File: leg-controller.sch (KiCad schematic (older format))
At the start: 15 parts, among them J1 Conn_01x02, J2 Conn_01x03, U1 LD1117S33TR_SOT223, U2 ATmega644P-20AU, Y1 12MHz

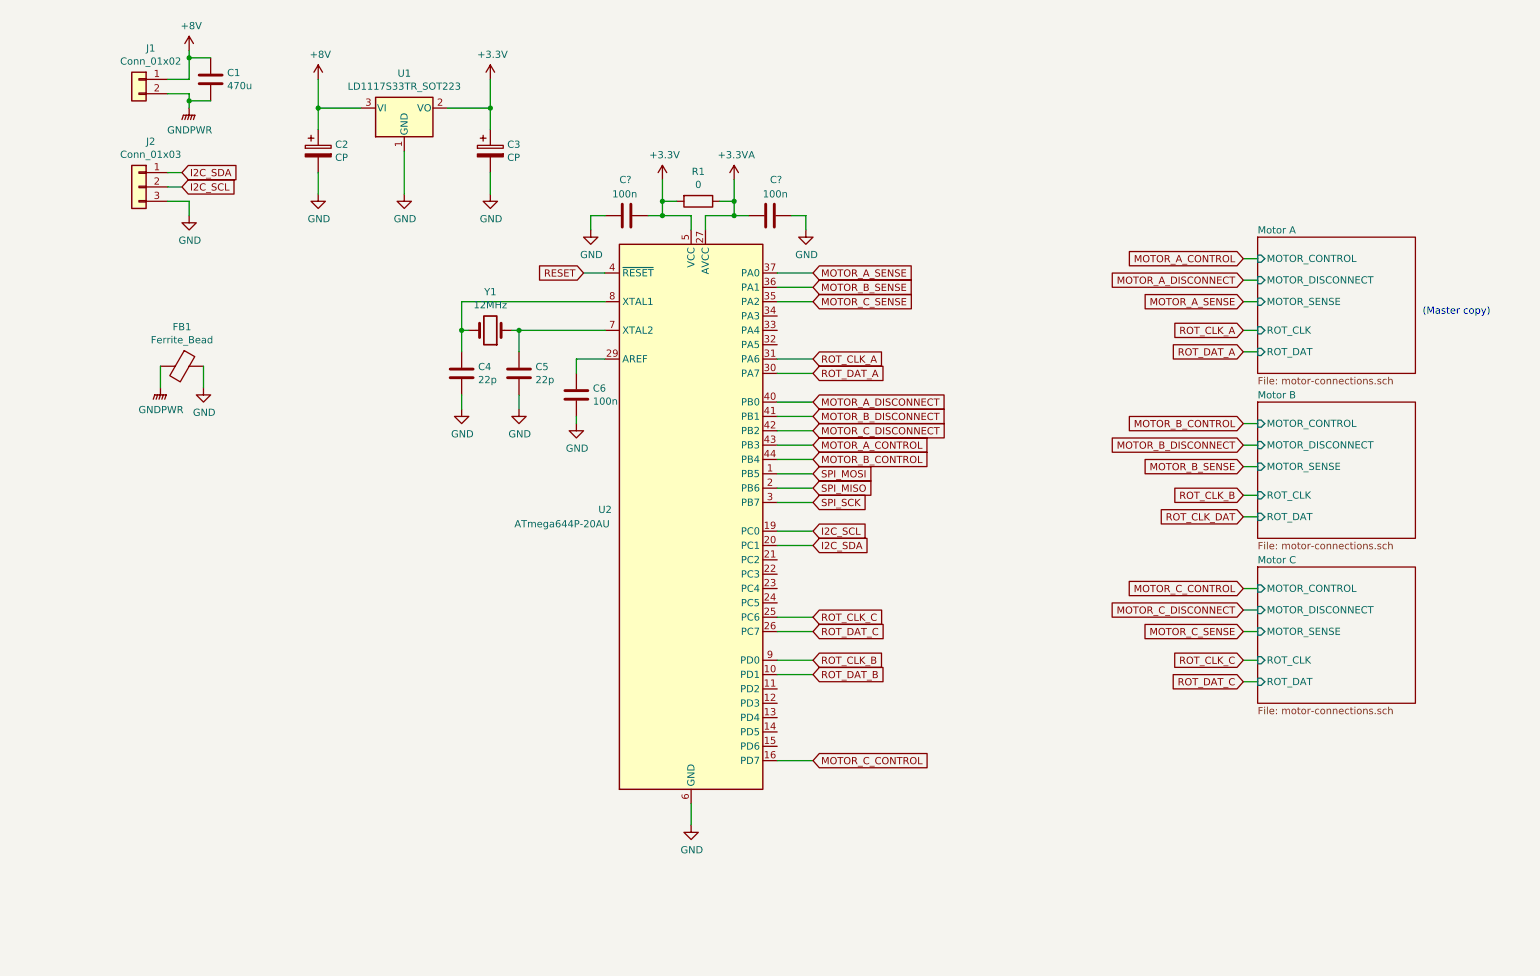
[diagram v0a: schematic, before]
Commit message: Various changes
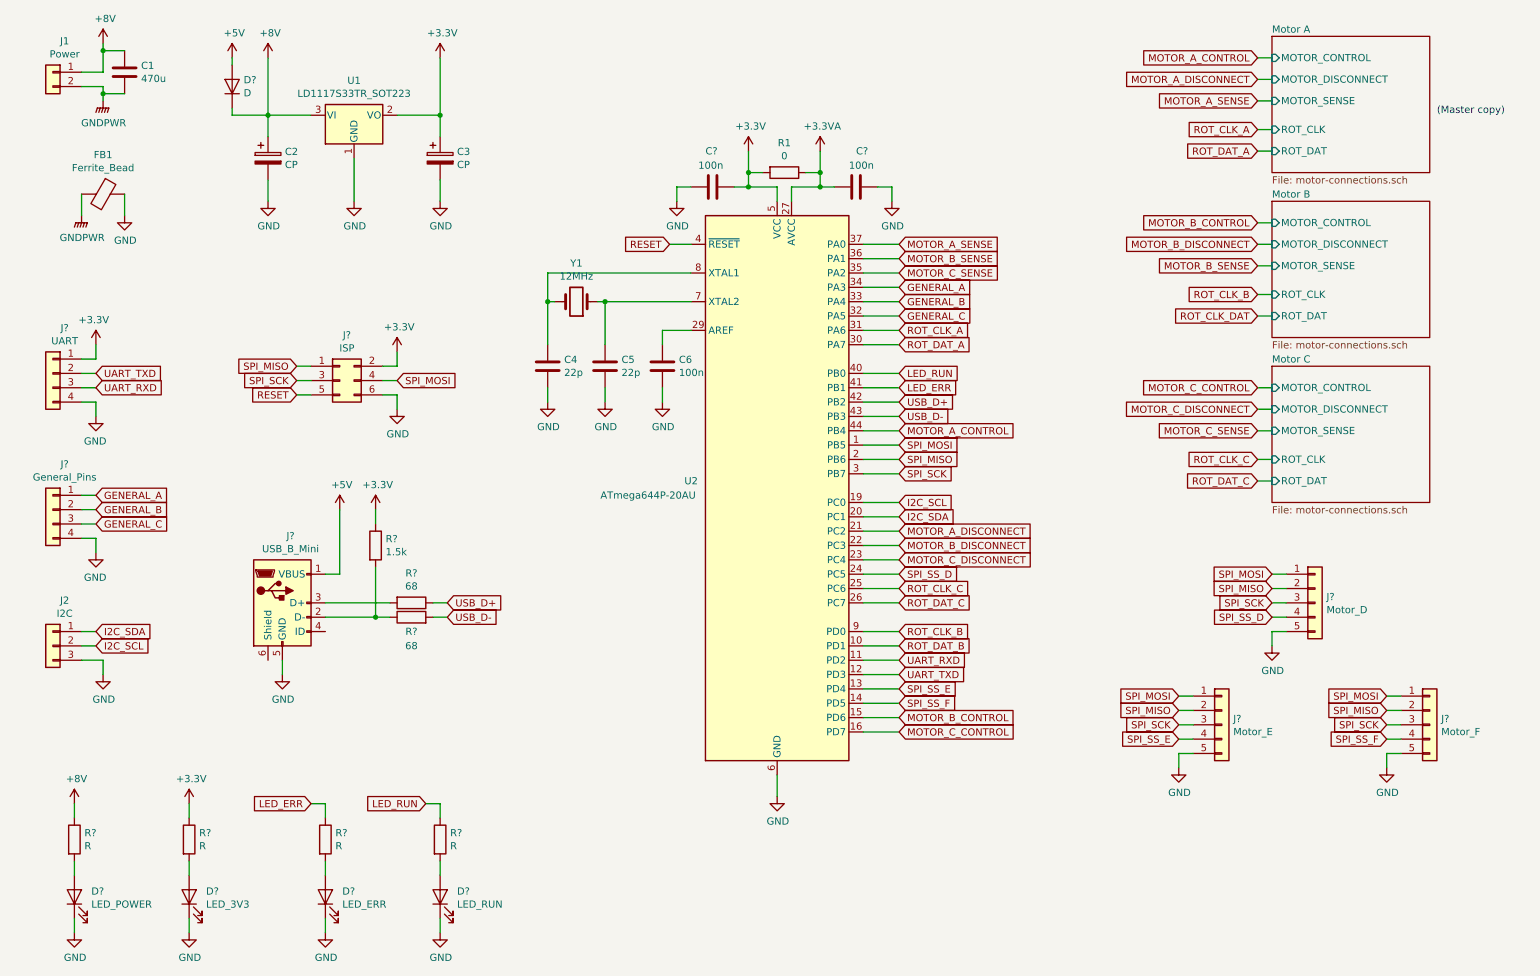
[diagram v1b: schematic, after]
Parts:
- added D?: LED_RUN, symbol Device:LED
- added D?: LED_POWER, symbol Device:LED
- added D?: LED_3V3, symbol Device:LED
- added D?: LED_ERR, symbol Device:LED
- added D?: D, symbol Device:D
- added J?: Motor_D, symbol Connector_Generic:Conn_01x05
- added J?: Motor_F, symbol Connector_Generic:Conn_01x05
- added J?: Motor_E, symbol Connector_Generic:Conn_01x05
- added J?: ISP, symbol Connector_Generic:Conn_02x03_Odd_Even
- added J?: UART, symbol Connector_Generic:Conn_01x04
- added J?: General_Pins, symbol Connector_Generic:Conn_01x04
- added J?: USB_B_Mini, symbol Connector:USB_B_Mini
- added R? (x4): R, symbol Device:R
- added R? (x2): 68, symbol Device:R
- added R?: 1.5k, symbol Device:R
- J1: value Conn_01x02 -> Power
- J2: value Conn_01x03 -> I2C
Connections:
- net +3V3: now also J?.1 (Pin_1), J?.2 (Pin_2), R?.1, R?.1
- net +8V: now also D?.1 (K), R?.1
- net GND: now also D?.1 (K), D?.1 (K), D?.1 (K), D?.1 (K), J?.4 (Pin_4), J?.4 (Pin_4), J?.5 (GND), J?.5 (Pin_5), J?.5 (Pin_5), J?.5 (Pin_5), J?.6 (Pin_6)
- net MOTOR_A_CONTROL: now also U2.44 (PB4); no longer U2.43 (PB3)
- net MOTOR_A_DISCONNECT: now also U2.21 (PC2); no longer U2.40 (PB0)
- net MOTOR_B_CONTROL: now also U2.15 (PD6); no longer U2.44 (PB4)
- net MOTOR_B_DISCONNECT: now also U2.22 (PC3); no longer U2.41 (PB1)
- net MOTOR_C_DISCONNECT: now also U2.23 (PC4); no longer U2.42 (PB2)
- net RESET: now also J?.5 (Pin_5)
- net SPI_MISO: now also J?.1 (Pin_1), J?.2 (Pin_2), J?.2 (Pin_2), J?.2 (Pin_2)
- net SPI_MOSI: now also J?.1 (Pin_1), J?.1 (Pin_1), J?.1 (Pin_1), J?.4 (Pin_4)
- net SPI_SCK: now also J?.3 (Pin_3), J?.3 (Pin_3), J?.3 (Pin_3), J?.3 (Pin_3)
- net UART_RXD: now reaches U2.11 (PD2)
- net UART_RXD: now also J?.3 (Pin_3)
- net UART_TXD: now reaches U2.12 (PD3)
- net UART_TXD: now also J?.2 (Pin_2)
- net SPI_SS_E: now reaches U2.13 (PD4)
- net SPI_SS_E: now also J?.4 (Pin_4)
- net SPI_SS_F: now reaches U2.14 (PD5)
- net SPI_SS_F: now also J?.4 (Pin_4)
- net SPI_SS_D: now reaches U2.24 (PC5)
- net SPI_SS_D: now also J?.4 (Pin_4)
- net GENERAL_C: now reaches U2.32 (PA5)
- net GENERAL_C: now also J?.3 (Pin_3)
- net GENERAL_B: now reaches U2.33 (PA4)
- net GENERAL_B: now also J?.2 (Pin_2)
- net GENERAL_A: now reaches U2.34 (PA3)
- net GENERAL_A: now also J?.1 (Pin_1)
- new net: D?.2 (A), R?.2 (x4)
- new net: J?.2 (D-), R?.1, R?.2
- new net: J?.3 (D+), R?.2
- new net +5V: D?.2 (A), J?.1 (VBUS)
- new net LED_ERR: R?.1, U2.41 (PB1)
- new net LED_RUN: R?.1, U2.40 (PB0)
- new net USB_D+: R?.1, U2.42 (PB2)
- new net USB_D-: R?.2, U2.43 (PB3)
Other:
- moved on the sheet: C1, C2, C3, C4, C5, C6, C?, FB1, J1, J2, R1, U1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

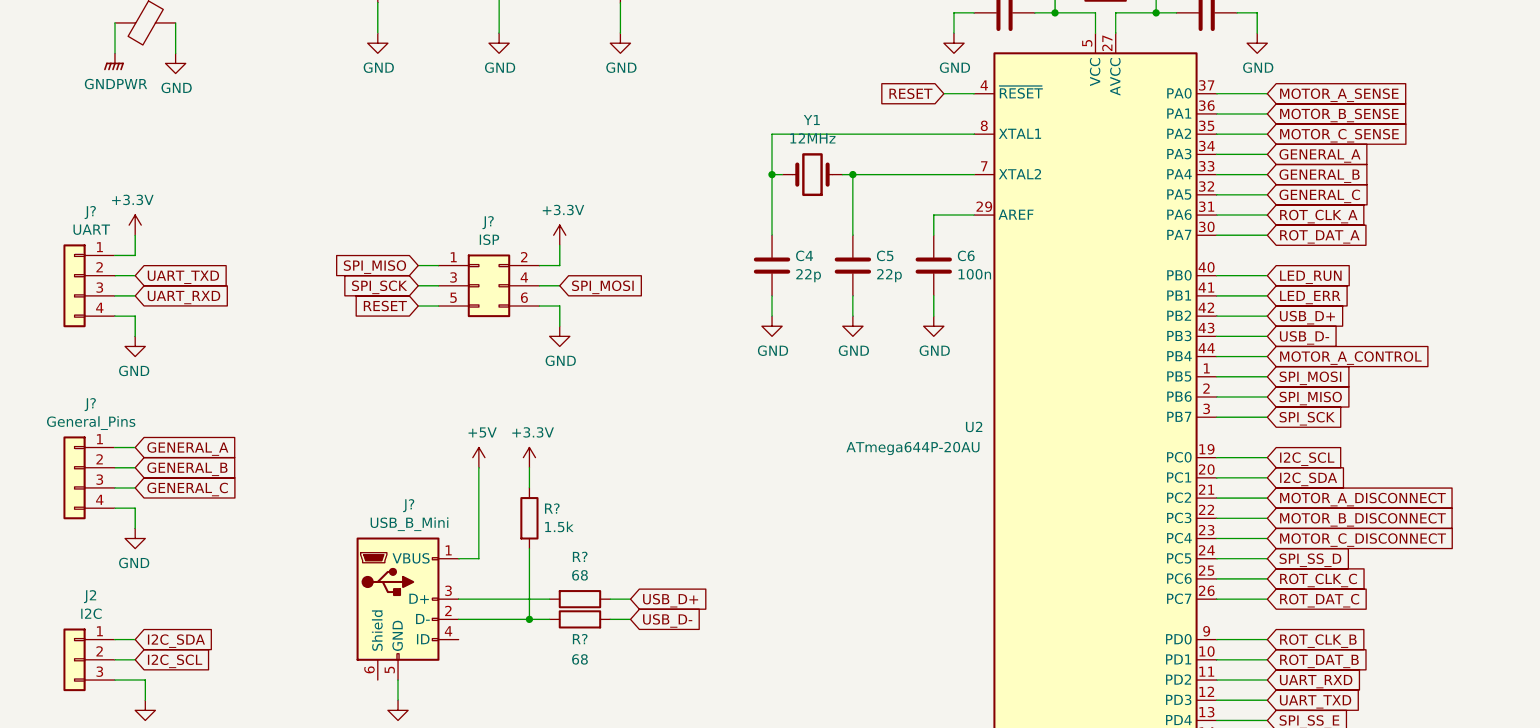
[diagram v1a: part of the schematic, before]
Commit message: Various changes.
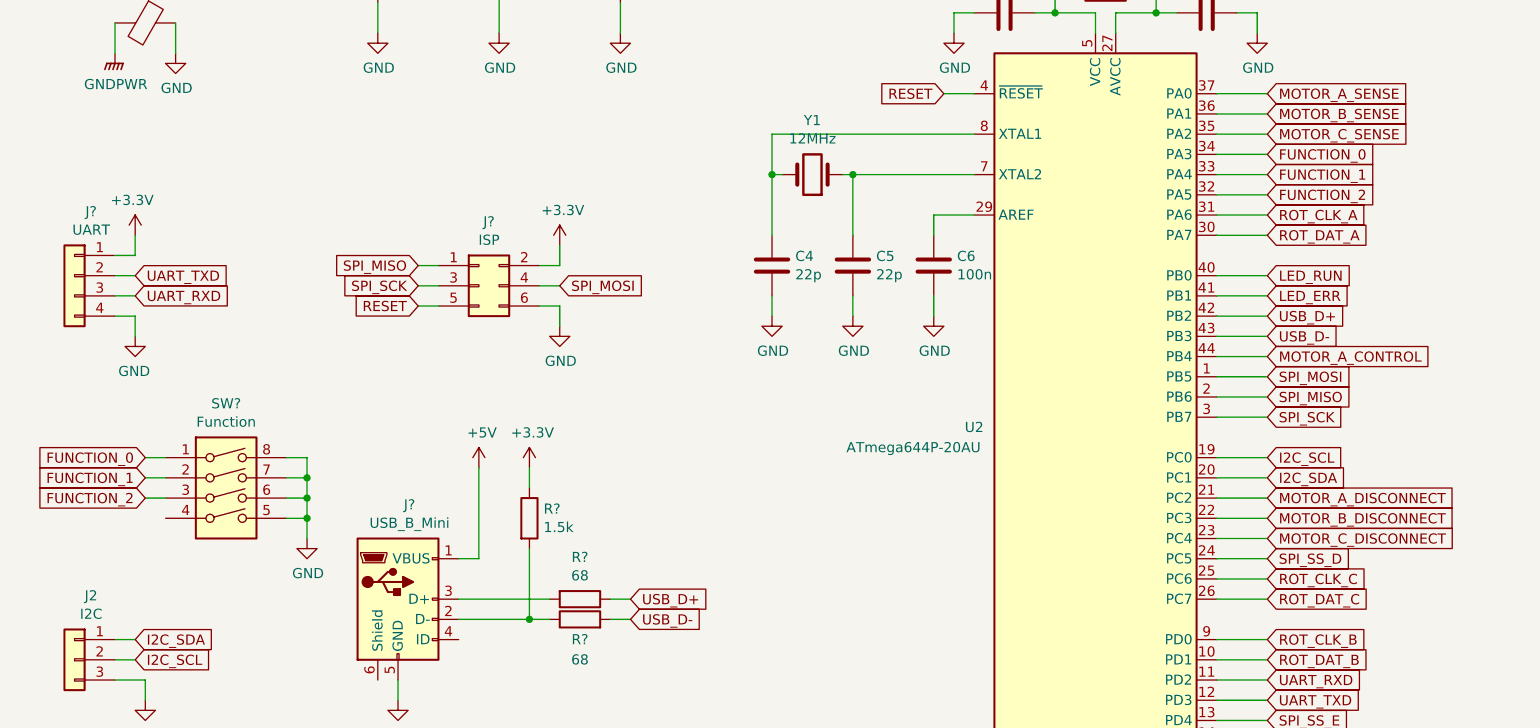
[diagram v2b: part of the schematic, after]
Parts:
- removed J?: General_Pins, symbol Connector_Generic:Conn_01x04
- added SW?: Function, symbol Switch:SW_DIP_x04
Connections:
- net GND: now also SW?.5, SW?.6, SW?.7, SW?.8
- net GENERAL_A renamed FUNCTION_0
- net FUNCTION_0: now also SW?.1
- net GENERAL_B renamed FUNCTION_1
- net FUNCTION_1: now also SW?.2
- net GENERAL_C renamed FUNCTION_2
- net FUNCTION_2: now also SW?.3
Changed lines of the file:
@@
 Wire Wire Line
 	3150 3250 3250 3250
-Text GLabel 1150 4050 2    50   Input ~ 0
-GENERAL_A
-Text GLabel 1150 4150 2    50   Input ~ 0
-GENERAL_B
-Text GLabel 1150 4250 2    50   Input ~ 0
-GENERAL_C
-Wire Wire Line
-	1150 4050 1050 4050
-Wire Wire Line
-	1050 4150 1150 4150
-Wire Wire Line
-	1150 4250 1050 4250
-$Comp
-L power:GND #PWR?
-U 1 1 61C68C47
-P 1150 4450
-F 0 "#PWR?" H 1150 4200 50  0001 C CNN
-F 1 "GND" H 1155 4277 50  0000 C CNN
-F 2 "" H 1150 4450 50  0001 C CNN
-F 3 "" H 1150 4450 50  0001 C CNN
-	1    1150 4450
-	-1   0    0    -1
-$EndComp
-Wire Wire Line
-	1150 4450 1150 4350
-Wire Wire Line
-	1150 4350 1050 4350
 $Comp
 L power:+5V #PWR?
@@
 $Comp
 L Connector_Generic:Conn_01x04 J?
-U 1 1 61C5169E
-P 850 4150
-F 0 "J?" H 768 4467 50  0000 C CNN
-F 1 "General_Pins" H 768 4376 50  0000 C CNN
-F 2 "" H 850 4150 50  0001 C CNN
-F 3 "~" H 850 4150 50  0001 C CNN
-	1    850  4150
-	-1   0    0    -1
-$EndComp
-$Comp
-L power:GND #PWR04
-U 1 1 6179673C
-P 1200 5300
-F 0 "#PWR04" H 1200 5050 50  0001 C CNN
-F 1 "GND" H 1205 5127 50  0000 C CNN
-F 2 "" H 1200 5300 50  0001 C CNN
-F 3 "" H 1200 5300 50  0001 C CNN
-	1    1200 5300
-	1    0    0    -1
-$EndComp
-Wire Wire Line
-	1200 5200 1200 5300
-Wire Wire Line
-	1050 5200 1200 5200
-Wire Wire Line
-	1050 5000 1150 5000
-Wire Wire Line
-	1050 5100 1150 5100
-Text GLabel 1150 5000 2    50   Input ~ 0
-I2C_SDA
-Text GLabel 1150 5100 2    50   Input ~ 0
-I2C_SCL
-$Comp
-L Connector_Generic:Conn_01x03 J2
-U 1 1 61793AA3
-P 850 5100
-F 0 "J2" H 768 5417 50  0000 C CNN
-F 1 "I2C" H 768 5326 50  0000 C CNN
-F 2 "" H 850 5100 50  0001 C CNN
-F 3 "~" H 850 5100 50  0001 C CNN
-	1    850  5100
-	-1   0    0    -1
-$EndComp
-$Comp
-L Connector_Generic:Conn_01x04 J?
 U 1 1 61B3D105
 P 850 3200
@@
 Wire Wire Line
 	1050 3200 1150 3200
-$Comp
-L Connector:USB_B_Mini J?
-U 1 1 61C85C74
-P 2450 4800
-F 0 "J?" H 2507 5267 50  0000 C CNN
-F 1 "USB_B_Mini" H 2507 5176 50  0000 C CNN
-F 2 "" H 2600 4750 50  0001 C CNN
-F 3 "~" H 2600 4750 50  0001 C CNN
-	1    2450 4800
-	1    0    0    -1
-$EndComp
-$Comp
-L Device:R R?
-U 1 1 61C9C39E
-P 3350 4800
-F 0 "R?" V 3143 4800 50  0000 C CNN
-F 1 "68" V 3234 4800 50  0000 C CNN
-F 2 "" V 3280 4800 50  0001 C CNN
-F 3 "~" H 3350 4800 50  0001 C CNN
-	1    3350 4800
-	0    1    1    0
-$EndComp
-$Comp
-L Device:R R?
-U 1 1 61C9D08A
-P 3350 4900
-F 0 "R?" V 3250 4900 50  0000 C CNN
-F 1 "68" V 3150 4900 50  0000 C CNN
-F 2 "" V 3280 4900 50  0001 C CNN
-F 3 "~" H 3350 4900 50  0001 C CNN
-	1    3350 4900
-	0    -1   -1   0
-$EndComp
-$Comp
-L Device:R R?
-U 1 1 61CB53AC
-P 3100 4400
-F 0 "R?" H 3170 4446 50  0000 L CNN
-F 1 "1.5k" H 3170 4355 50  0000 L CNN
-F 2 "" V 3030 4400 50  0001 C CNN
-F 3 "~" H 3100 4400 50  0001 C CNN
-	1    3100 4400
-	1    0    0    -1
-$EndComp
-Wire Wire Line
-	3100 4550 3100 4900
-Connection ~ 3100 4900
-Wire Wire Line
-	3100 4900 3200 4900
-$Comp
-L power:+3.3V #PWR?
-U 1 1 61CBCED0
-P 3100 4150
-F 0 "#PWR?" H 3100 4000 50  0001 C CNN
-F 1 "+3.3V" H 3115 4323 50  0000 C CNN
-F 2 "" H 3100 4150 50  0001 C CNN
-F 3 "" H 3100 4150 50  0001 C CNN
-	1    3100 4150
-	1    0    0    -1
-$EndComp
-Wire Wire Line
-	3100 4150 3100 4250
-$Comp
-L power:GND #PWR?
-U 1 1 61CC49B7
-P 2450 5300
-F 0 "#PWR?" H 2450 5050 50  0001 C CNN
-F 1 "GND" H 2455 5127 50  0000 C CNN
-F 2 "" H 2450 5300 50  0001 C CNN
-F 3 "" H 2450 5300 50  0001 C CNN
-	1    2450 5300
-	1    0    0    -1
-$EndComp
-Wire Wire Line
-	2450 5200 2450 5300
-Wire Wire Line
-	3600 4800 3500 4800
-Wire Wire Line
-	3500 4900 3600 4900
-$Comp
-L power:+5V #PWR?
-U 1 1 61D1E6C0
-P 2850 4150
-F 0 "#PWR?" H 2850 4000 50  0001 C CNN
-F 1 "+5V" H 2865 4323 50  0000 C CNN
-F 2 "" H 2850 4150 50  0001 C CNN
-F 3 "" H 2850 4150 50  0001 C CNN
-	1    2850 4150
-	1    0    0    -1
-$EndComp
-Wire Wire Line
-	2750 4600 2850 4600
-Wire Wire Line
-	2850 4600 2850 4150
-Wire Wire Line
-	2750 4800 3200 4800
-Wire Wire Line
-	2750 4900 3100 4900
 Wire Wire Line
 	3550 6200 3450 6200
@@
 	6500 5200 6750 5200
 Text GLabel 6750 2600 2    50   Input ~ 0
-GENERAL_A
+FUNCTION_0
 Text GLabel 6750 2700 2    50   Input ~ 0
-GENERAL_B
+FUNCTION_1
 Text GLabel 6750 2800 2    50   Input ~ 0
-GENERAL_C
+FUNCTION_2
 Wire Wire Line
 	6750 2600 6500 2600
@@
 Wire Wire Line
 	4700 2700 5300 2700
+Text GLabel 3600 4800 2    50   Input ~ 0
+USB_D+
 Text GLabel 3600 4900 2    50   Input ~ 0
 USB_D-
-Text GLabel 3600 4800 2    50   Input ~ 0
-USB_D+
+Wire Wire Line
+	2750 4900 3100 4900
+Wire Wire Line
+	2750 4800 3200 4800
+Wire Wire Line
+	2850 4600 2850 4150
+Wire Wire Line
+	2750 4600 2850 4600
+$Comp
+L power:+5V #PWR?
+U 1 1 61D1E6C0
+P 2850 4150
+F 0 "#PWR?" H 2850 4000 50  0001 C CNN
+F 1 "+5V" H 2865 4323 50  0000 C CNN
+F 2 "" H 2850 4150 50  0001 C CNN
+F 3 "" H 2850 4150 50  0001 C CNN
+	1    2850 4150
+	1    0    0    -1
+$EndComp
+Wire Wire Line
+	3500 4900 3600 4900
+Wire Wire Line
+	3600 4800 3500 4800
+Wire Wire Line
+	2450 5200 2450 5300
+$Comp
+L power:GND #PWR?
+U 1 1 61CC49B7
+P 2450 5300
+F 0 "#PWR?" H 2450 5050 50  0001 C CNN
+F 1 "GND" H 2455 5127 50  0000 C CNN
+F 2 "" H 2450 5300 50  0001 C CNN
+F 3 "" H 2450 5300 50  0001 C CNN
+	1    2450 5300
+	1    0    0    -1
+$EndComp
+Wire Wire Line
+	3100 4150 3100 4250
+$Comp
+L power:+3.3V #PWR?
+U 1 1 61CBCED0
+P 3100 4150
+F 0 "#PWR?" H 3100 4000 50  0001 C CNN
+F 1 "+3.3V" H 3115 4323 50  0000 C CNN
+F 2 "" H 3100 4150 50  0001 C CNN
+F 3 "" H 3100 4150 50  0001 C CNN
+	1    3100 4150
+	1    0    0    -1
+$EndComp
+Wire Wire Line
+	3100 4900 3200 4900
+Connection ~ 3100 4900
+Wire Wire Line
+	3100 4550 3100 4900
+$Comp
+L Device:R R?
+U 1 1 61CB53AC
+P 3100 4400
+F 0 "R?" H 3170 4446 50  0000 L CNN
+F 1 "1.5k" H 3170 4355 50  0000 L CNN
+F 2 "" V 3030 4400 50  0001 C CNN
+F 3 "~" H 3100 4400 50  0001 C CNN
+	1    3100 4400
+	1    0    0    -1
+$EndComp
+$Comp
+L Device:R R?
+U 1 1 61C9D08A
+P 3350 4900
+F 0 "R?" V 3250 4900 50  0000 C CNN
+F 1 "68" V 3150 4900 50  0000 C CNN
+F 2 "" V 3280 4900 50  0001 C CNN
+F 3 "~" H 3350 4900 50  0001 C CNN
+	1    3350 4900
+	0    -1   -1   0
+$EndComp
+$Comp
+L Device:R R?
+U 1 1 61C9C39E
+P 3350 4800
+F 0 "R?" V 3143 4800 50  0000 C CNN
+F 1 "68" V 3234 4800 50  0000 C CNN
+F 2 "" V 3280 4800 50  0001 C CNN
+F 3 "~" H 3350 4800 50  0001 C CNN
+	1    3350 4800
+	0    1    1    0
+$EndComp
+$Comp
+L Connector:USB_B_Mini J?
+U 1 1 61C85C74
+P 2450 4800
+F 0 "J?" H 2507 5267 50  0000 C CNN
+F 1 "USB_B_Mini" H 2507 5176 50  0000 C CNN
+F 2 "" H 2600 4750 50  0001 C CNN
+F 3 "~" H 2600 4750 50  0001 C CNN
+	1    2450 4800
+	1    0    0    -1
+$EndComp
+$Comp
+L Connector_Generic:Conn_01x03 J2
+U 1 1 61793AA3
+P 850 5100
+F 0 "J2" H 768 5417 50  0000 C CNN
+F 1 "I2C" H 768 5326 50  0000 C CNN
+F 2 "" H 850 5100 50  0001 C CNN
+F 3 "~" H 850 5100 50  0001 C CNN
+	1    850  5100
+	-1   0    0    -1
+$EndComp
+Text GLabel 1150 5100 2    50   Input ~ 0
+I2C_SCL
+Text GLabel 1150 5000 2    50   Input ~ 0
+I2C_SDA
+Wire Wire Line
+	1050 5100 1150 5100
+Wire Wire Line
+	1050 5000 1150 5000
+Wire Wire Line
+	1050 5200 1200 5200
+Wire Wire Line
+	1200 5200 1200 5300
+$Comp
+L power:GND #PWR04
+U 1 1 6179673C
+P 1200 5300
+F 0 "#PWR04" H 1200 5050 50  0001 C CNN
+F 1 "GND" H 1205 5127 50  0000 C CNN
+F 2 "" H 1200 5300 50  0001 C CNN
+F 3 "" H 1200 5300 50  0001 C CNN
+	1    1200 5300
+	1    0    0    -1
+$EndComp
+Wire Wire Line
+	1200 4300 1300 4300
+Wire Wire Line
+	1200 4200 1300 4200
+Wire Wire Line
+	1200 4100 1300 4100
+Text GLabel 1200 4300 0    50   Input ~ 0
+FUNCTION_2
+Text GLabel 1200 4200 0    50   Input ~ 0
+FUNCTION_1
+Text GLabel 1200 4100 0    50   Input ~ 0
+FUNCTION_0
+Wire Wire Line
+	2000 4400 2000 4500
+Connection ~ 2000 4400
+Wire Wire Line
+	1900 4400 2000 4400
+Wire Wire Line
+	2000 4300 2000 4400
+Connection ~ 2000 4300
+Wire Wire Line
+	1900 4300 2000 4300
+Wire Wire Line
+	2000 4200 2000 4300
+Connection ~ 2000 4200
+Wire Wire Line
+	1900 4200 2000 4200
+Wire Wire Line
+	2000 4100 2000 4200
+Wire Wire Line
+	1900 4100 2000 4100
+$Comp
+L power:GND #PWR?
+U 1 1 6199B184
+P 2000 4500
+F 0 "#PWR?" H 2000 4250 50  0001 C CNN
+F 1 "GND" H 2005 4327 50  0000 C CNN
+F 2 "" H 2000 4500 50  0001 C CNN
+F 3 "" H 2000 4500 50  0001 C CNN
+	1    2000 4500
+	1    0    0    -1
+$EndComp
+$Comp
+L Switch:SW_DIP_x04 SW?
+U 1 1 6199597A
+P 1600 4300
+F 0 "SW?" H 1600 4767 50  0000 C CNN
+F 1 "Function" H 1600 4676 50  0000 C CNN
+F 2 "" H 1600 4300 50  0001 C CNN
+F 3 "~" H 1600 4300 50  0001 C CNN
+	1    1600 4300
+	1    0    0    -1
+$EndComp
 $EndSCHEMATC
